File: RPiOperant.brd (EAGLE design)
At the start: 136 x 100 mm, 62 parts, among them IC1 74LS14N, IC2 74LS14N, IC3 MCP3008, J1 USB_B_PTH, J2 POWER_JACK, J3 POWER_JACK, J4 USB_B_PTH, J5 1X2-3.5MM, J6 1X2-3.5MM, J7 1X2-3.5MM, J8 1X2-3.5MM, J9 1X2-3.5MM

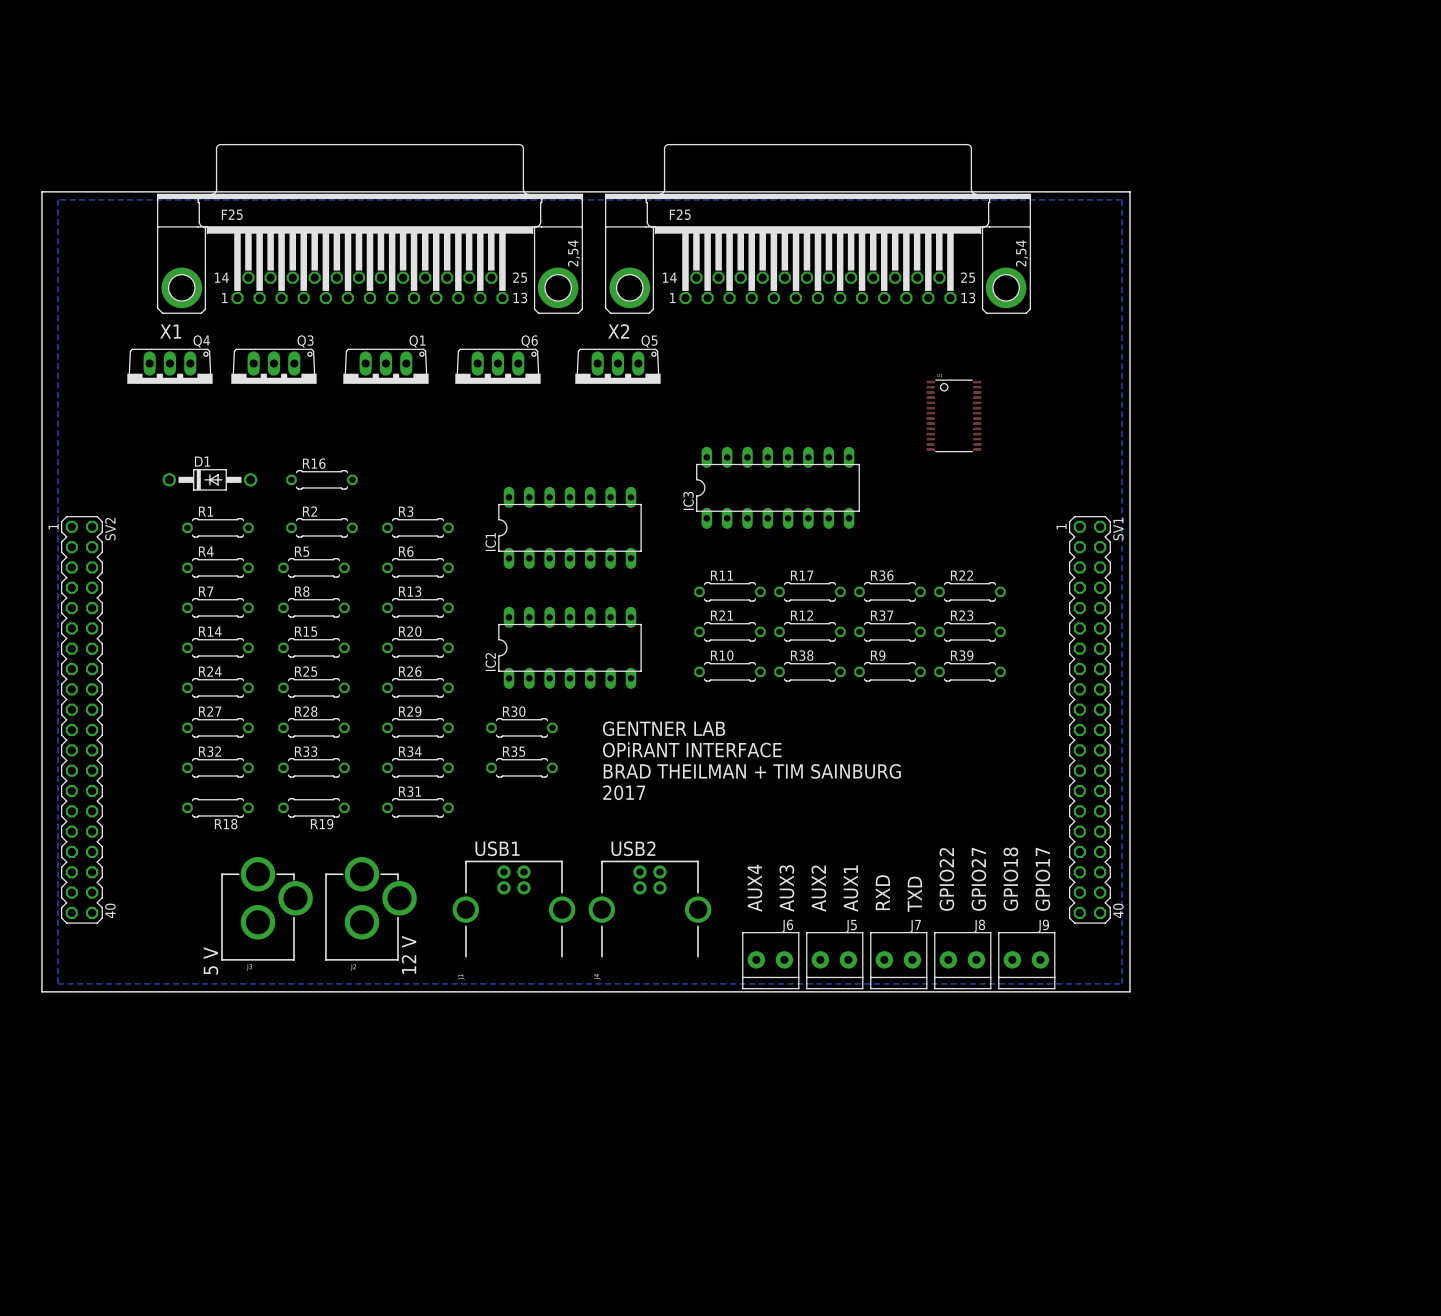
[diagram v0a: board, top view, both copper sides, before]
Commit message: new stuff!
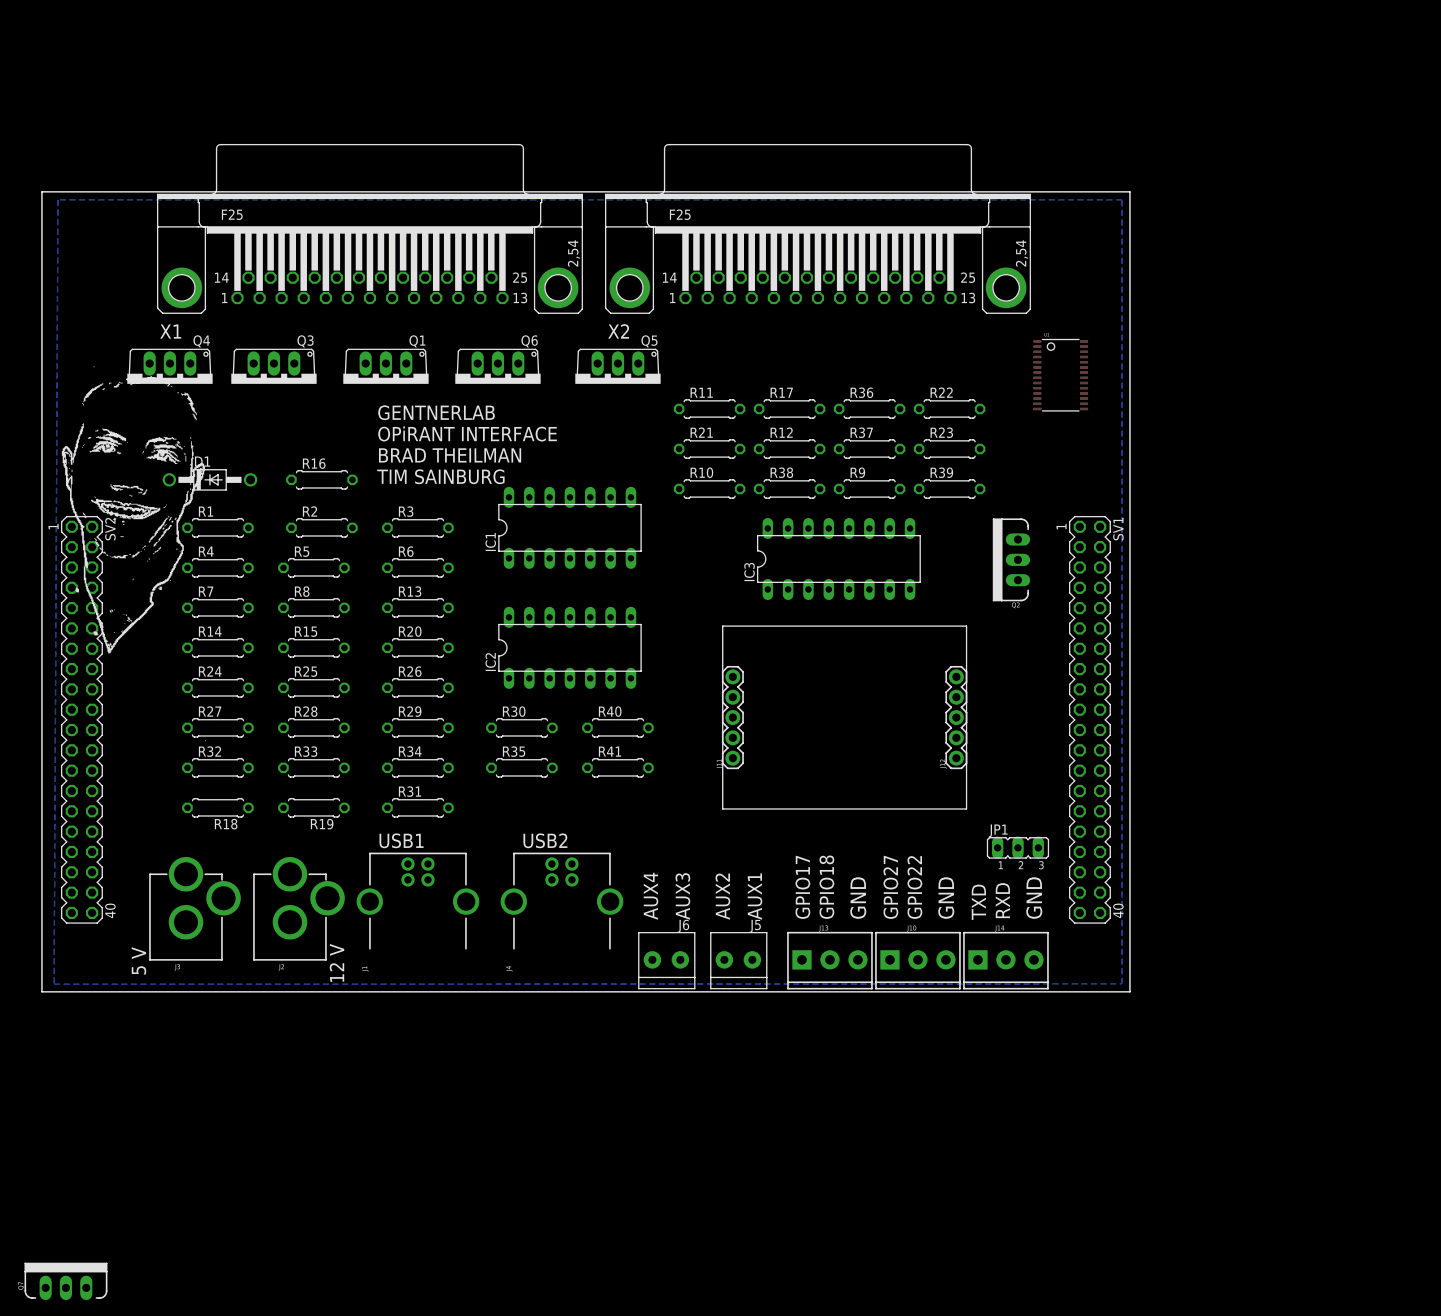
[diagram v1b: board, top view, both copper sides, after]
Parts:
- removed J7, J8, J9: 1X2-3.5MM, adafruit:1X2-3.5MM
- added J10, J13, J14: (no value), SparkFun-Connectors:SCREWTERMINAL-3.5MM-3
- added J11, J12: (no value), SparkFun-Connectors:1X05
- added JP1: (no value), jumper:JP2
- added Q2, Q7: 60V/32A/35mΩ, SparkFun-DiscreteSemi:TO220V
- added R40, R41: 10K, resistor:0207/7
- moved R10 23.0 mm to (83.5, 62.9)
- moved R11 23.0 mm to (83.5, 72.9)
- moved R12 23.0 mm to (93.5, 67.9)
- moved R17 23.0 mm to (93.5, 72.9)
- moved R21 23.0 mm to (83.5, 67.9)
- moved R22 23.0 mm to (113.5, 72.9)
- moved R23 23.0 mm to (113.5, 67.9)
- moved R36 23.0 mm to (103.5, 72.9)
- moved R37 23.0 mm to (103.5, 67.9)
- moved R38 23.0 mm to (93.5, 62.9)
- moved R39 23.0 mm to (113.5, 62.9)
- moved R9 23.0 mm to (103.5, 62.9)
- moved U1 14.3 mm to (127.3, 77.1)
- moved J6 13.0 mm to (78.0, 4.00)
- moved J1 12.0 mm to (47.0, 10.0)
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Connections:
- removed net TEMP: X1.2
- new net DAT: J12.3
- new net LCCLK: J12.2
- new net TTL27: J10.1, Q2.2, R41.2
- new net YLW: J11.1
- net +3V3: now also J12.4
- net GND: now also J10.3, J12.1, J13.3, J14.3
- net GPIO17: now also J13.1; no longer J9.1
- net GPIO18: now also J13.2, X1.2; no longer J9.2
- net GPIO22: now also J10.2; no longer J8.2
- net GPIO27: now also Q2.3, R40.2; no longer J8.1
- net LOADCELLA+: now also J11.3
- net LOADCELLA-: now also J11.2
- net LOADCELLE+: now also J11.5
- net LOADCELLE-: now also J11.4
- net RPI_3.3V: now also JP1.1, Q2.1, R40.1
- net RPI_5V: now also JP1.2, JP1.3, R41.1
- net RXD: now also J14.2; no longer J7.2
- net TXD: now also J14.1; no longer J7.1
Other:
- board text added: "GENTNERLAB OPiRANT INTERFACE BRAD THEILMAN TIM SAINBURG"
- board text added: "GND"
- board text removed: "GENTNER LAB OPiRANT INTERFACE BRAD THEILMAN + TIM SAINBURG 2017"

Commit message: final draft
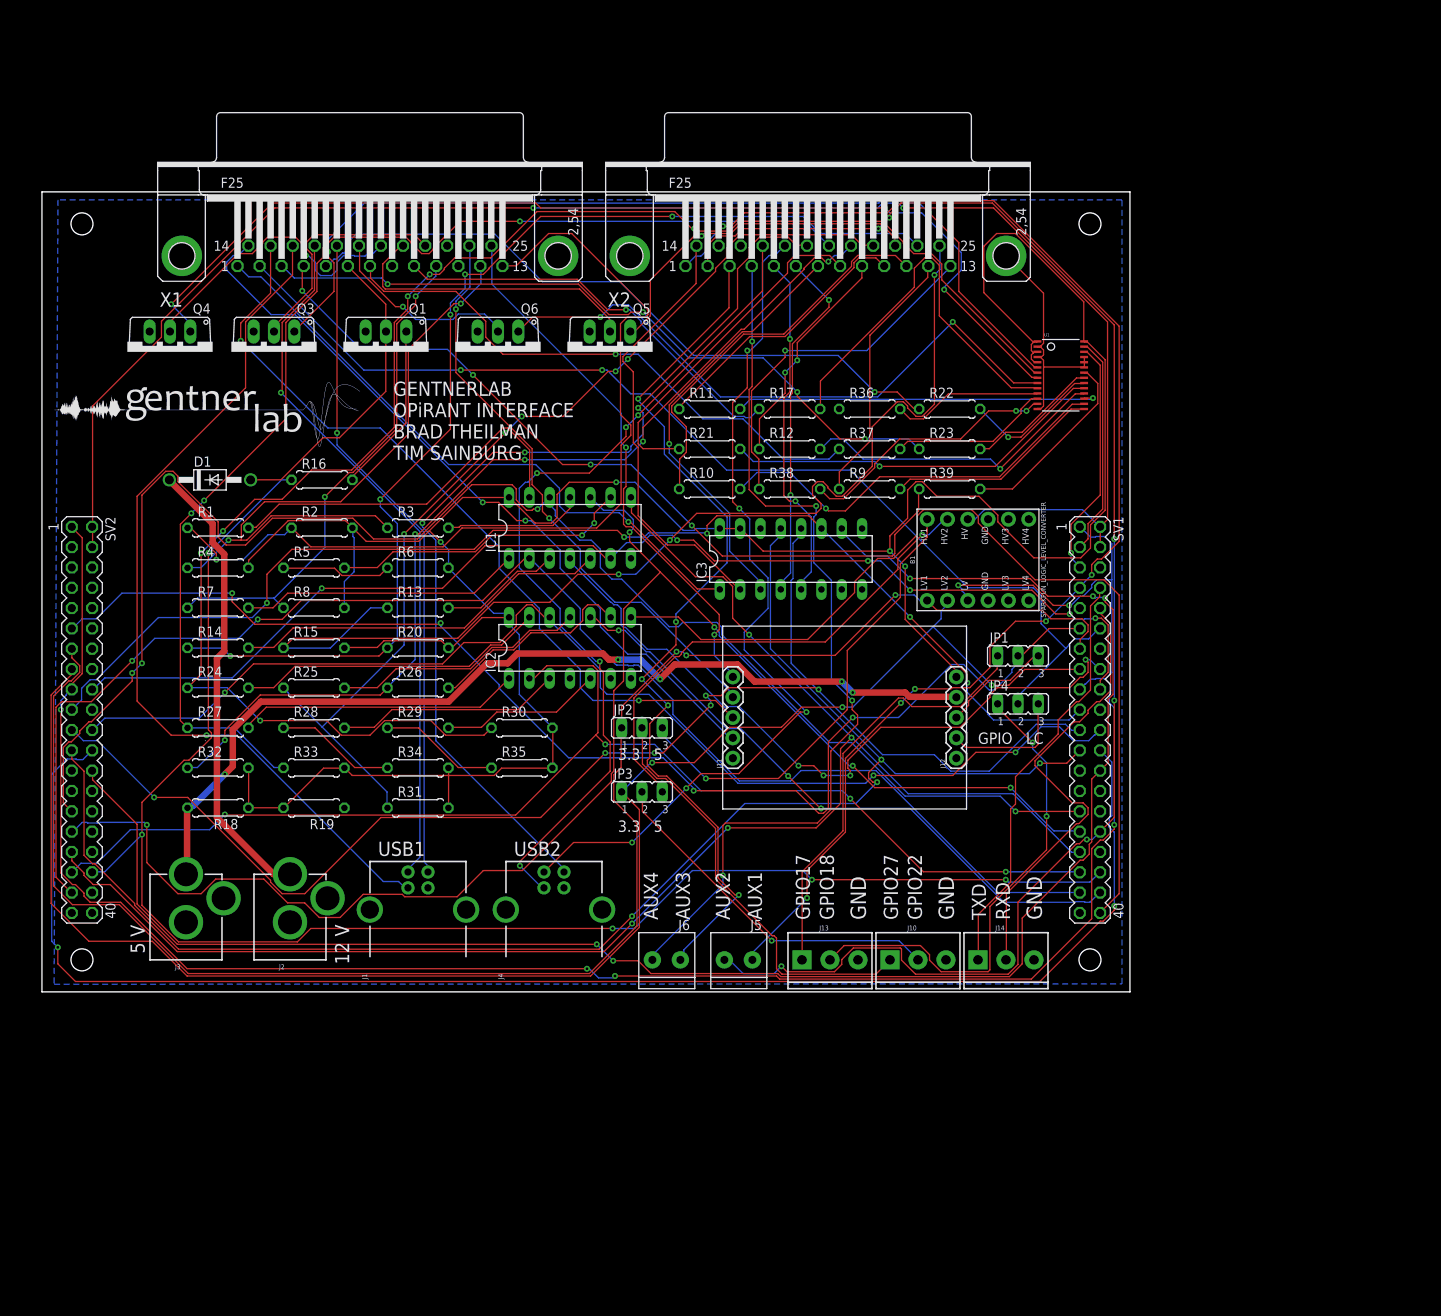
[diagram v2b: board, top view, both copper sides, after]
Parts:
- removed Q2, Q7: 60V/32A/35mΩ, SparkFun-DiscreteSemi:TO220V
- removed R40, R41: 10K, resistor:0207/7
- added B1: SPARKFUN_LOGIC_LEVEL_CONVERTER, SparkFun-Boards:SPARKFUN_LOGIC_LEVEL_CONVERTER
- added JP2, JP3, JP4: (no value), jumper:JP2
- moved JP1 24.0 mm to (122.0, 42.0)
- moved IC3 6.00 mm to (93.6, 54.1)
- moved Q5 4.12 mm to (71.0, 80.0)
- moved Q1 4.00 mm to (43.0, 80.0)
- moved Q3 4.00 mm to (29.0, 80.0)
- moved Q4 4.00 mm to (16.0, 80.0)
- moved Q6 4.00 mm to (57.0, 80.0)
- moved X1 4.00 mm to (41.0, 92.0)
- moved X2 4.00 mm to (97.0, 92.0)
- moved J4 1.41 mm to (64.0, 9.00)
- moved J1 1.00 mm to (47.0, 9.00)
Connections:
- new net N$22: B1.HV1, JP2.3
- new net N$23: B1.HV2, JP3.3
- new net N$32: J13.1, JP1.1
- new net N$33: J13.2, JP4.1
- new net TTL22: J10.2, JP3.2
- net +3V3: now also J12.5; no longer J12.4
- net +5V: now also J12.4
- net DAT: now also JP1.3
- net GND: now also B1.GND1, B1.GND2
- net GPIO17: now also JP1.2; no longer J13.1
- net GPIO18: now also JP4.2; no longer J13.2
- net GPIO22: now also B1.LV2, JP3.1; no longer J10.2
- net GPIO27: now also B1.LV1, JP2.1; no longer Q2.3, R40.2
- net LCCLK: now also JP4.3
- net RPI_3.3V: now also B1.LV; no longer JP1.1, Q2.1, R40.1
- net RPI_5V: now also B1.HV; no longer JP1.2, JP1.3, R41.1
- net TTL27: now also JP2.2; no longer Q2.2, R41.2
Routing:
- net +3V3: track 0.00 -> 341.3 mm, vias 0 -> 4
- net RPI_3.3V: track 0.00 -> 265.0 mm, vias 0 -> 6
- net CE1: track 0.00 -> 221.9 mm, vias 0 -> 5
- net GPIO27: track 0.00 -> 210.0 mm, vias 0 -> 3
- net RPI_5V: track 0.00 -> 208.9 mm, vias 0 -> 2
- net GPIO22: track 0.00 -> 201.8 mm, vias 0 -> 3
- net HOPPER_TRIG_GPIO: track 0.00 -> 197.0 mm, vias 0 -> 5
- net CENTER_PECK_GPIO: track 0.00 -> 196.5 mm, vias 0 -> 4
- net HOPPER_IR_GPIO: track 0.00 -> 196.1 mm, vias 0 -> 4
- net LEFT_PECK_GPIO: track 0.00 -> 194.3 mm, vias 0 -> 5
- net SCLK: track 0.00 -> 192.7 mm, vias 0 -> 4
- net AUX2: track 0.00 -> 190.2 mm, vias 0 -> 6
- net CE0: track 0.00 -> 188.1 mm, vias 0 -> 2
- net RIGHT_PECK_GPIO: track 0.00 -> 180.8 mm, vias 0 -> 2
- net IR_3: track 0.00 -> 176.7 mm, vias 0 -> 7
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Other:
- board text added: "/home/brad/Pictures/gentnerlab_logo_inverted.bmp"
- board text added: "3.3 5"
- board text added: "GPIO LC"
